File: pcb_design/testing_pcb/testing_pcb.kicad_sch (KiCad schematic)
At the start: 56 parts, among them J1 UART, J10 SOx, J11 Conn_01x04_Pin, J12 Conn_01x04_Pin, J2 ST-LINK Flasher, J3 batt_1x2, J5 INH/Lx, J6 gnd, J7 V, J8 out, SW1 SW_Push, SW2 SW_Push, U1 STM32G431CBTx, U2 AMS1117, U3 DRV8311H, U4 AS5600

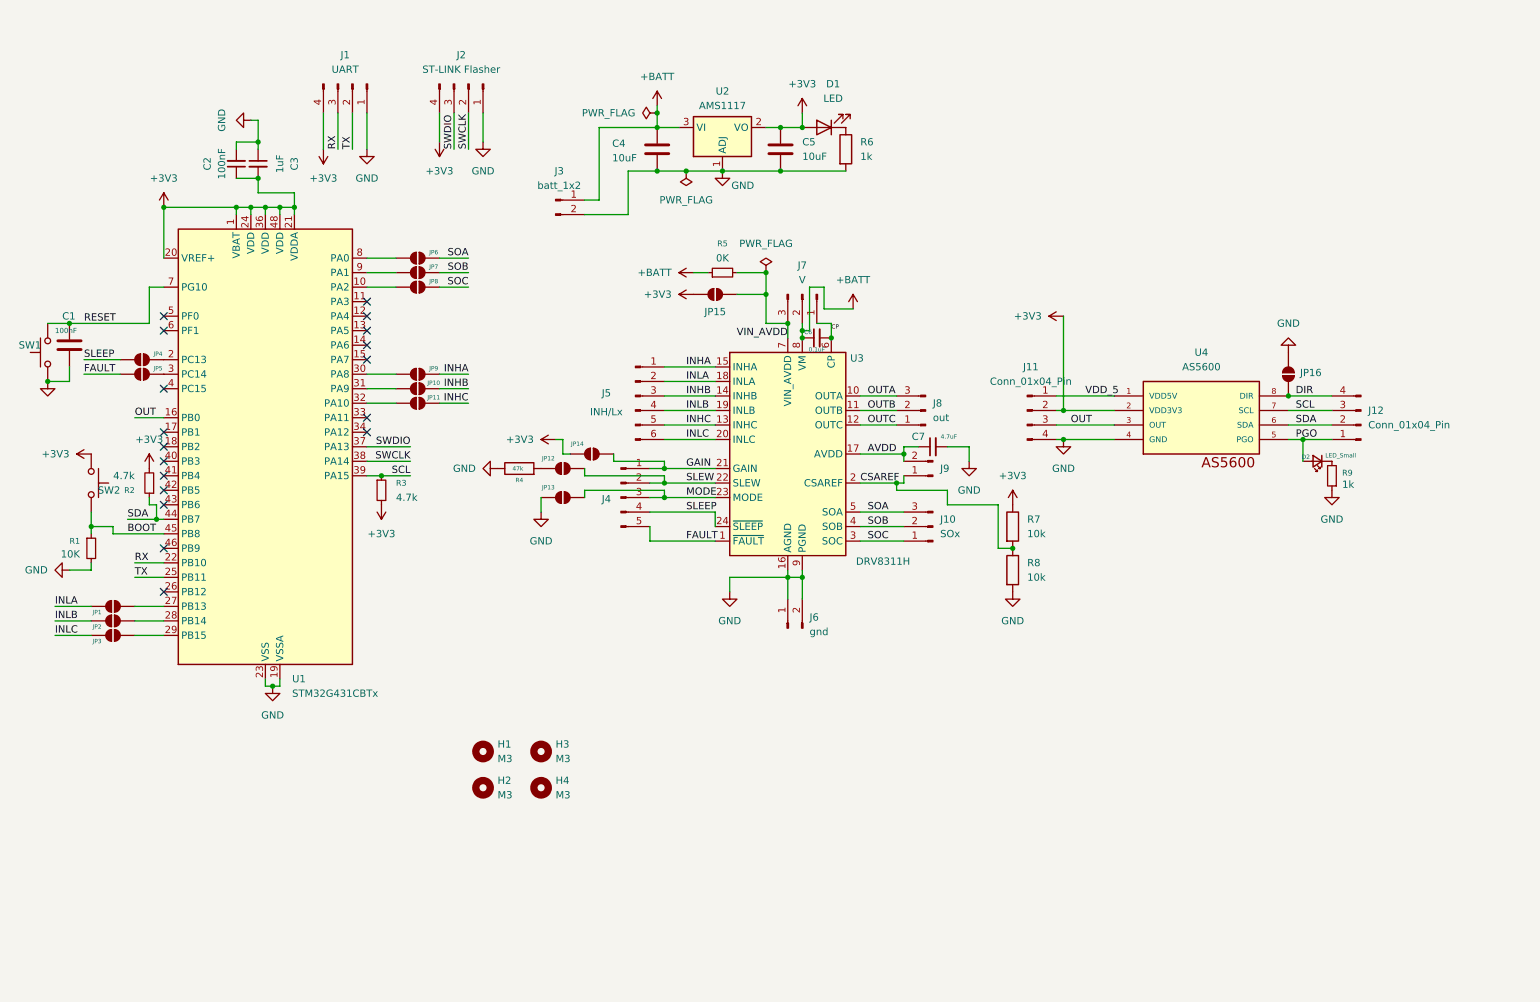
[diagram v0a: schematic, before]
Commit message: made schematic look good
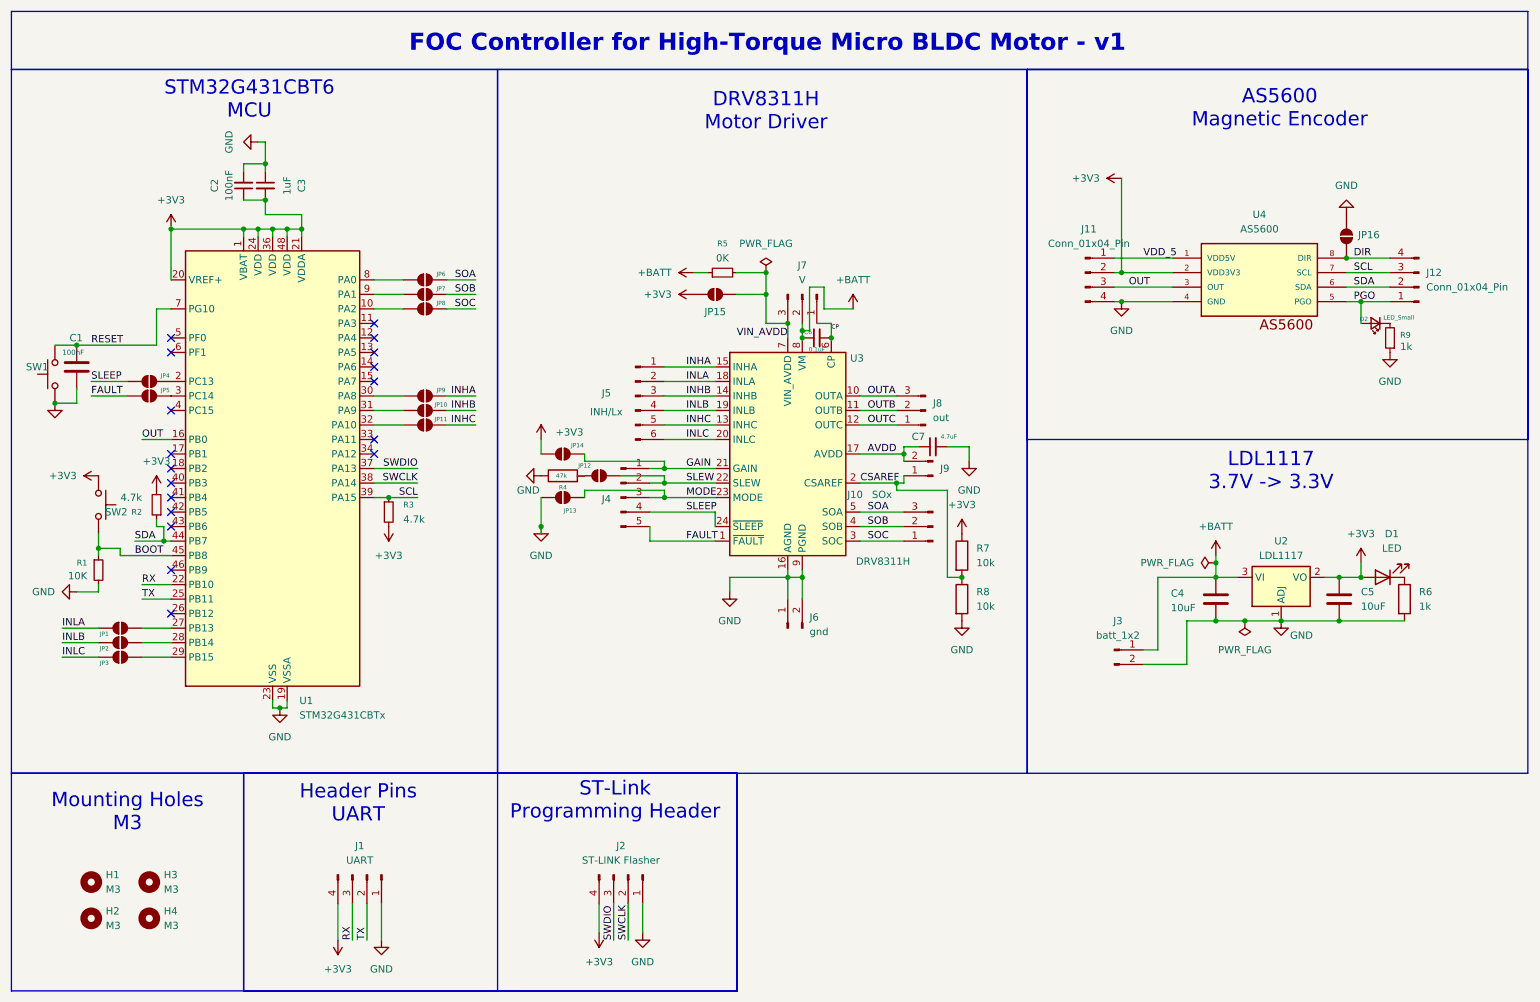
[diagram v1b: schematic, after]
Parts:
- U2: value AMS1117 -> LDL1117
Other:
- note added: "AS5600 Magnetic Encoder"
- note added: "DRV8311H Motor Driver"
- note added: "FOC Controller for High-Torque Micro BLDC Motor - v1"
- note added: "Header Pins UART"
- note added: "LDL1117 3.7V -> 3.3V"
- note added: "Mounting Holes M3"
- note added: "ST-Link Programming Header"
- note added: "STM32G431CBT6 MCU"
- moved on the sheet: C1, C2, C3, C4, C5, D1, D2, H1, H2, H3, H4, J1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
